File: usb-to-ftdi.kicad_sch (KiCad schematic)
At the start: 9 parts, among them J1 USB_OTG, J2 Conn_01x06, U1 AMS1117-3.3, U2 CH340C

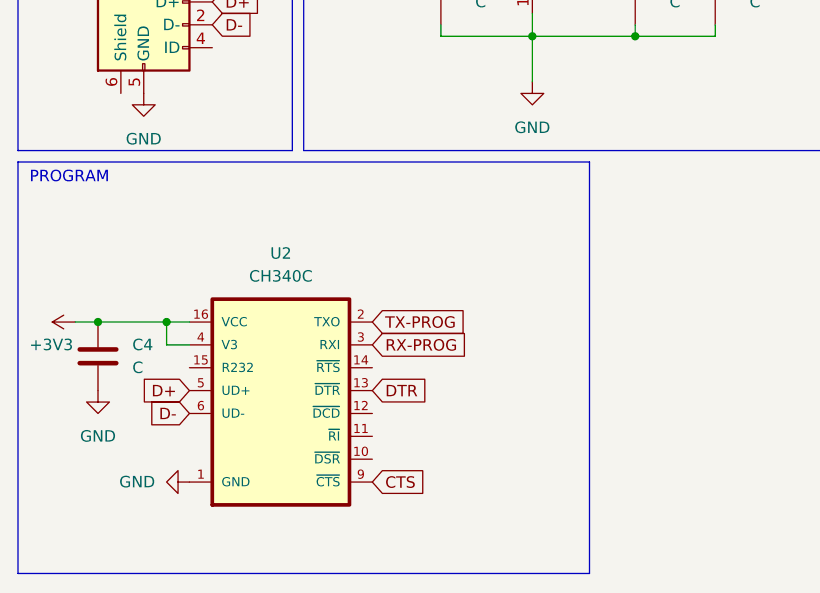
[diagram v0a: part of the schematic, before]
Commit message: add pcb + wiring
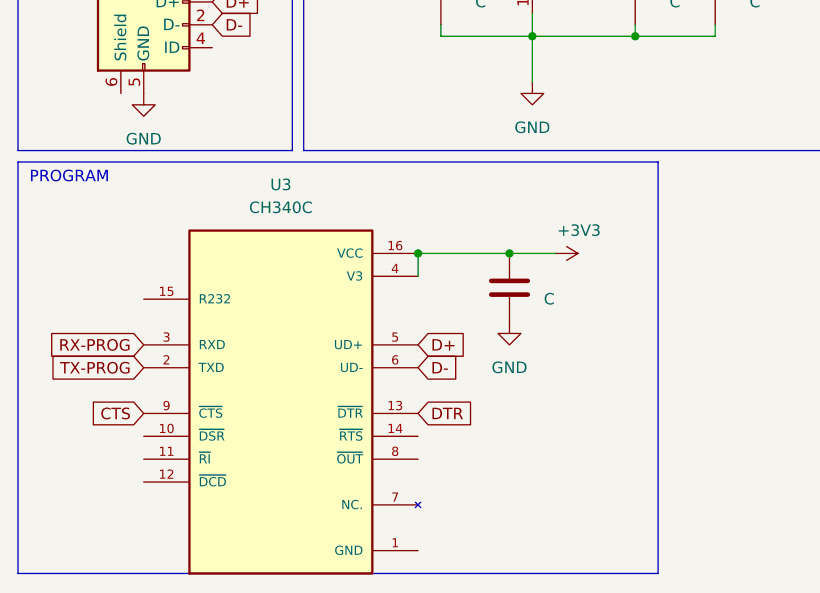
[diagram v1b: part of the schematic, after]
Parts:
- removed U2: CH340C, CH340C:SO016, symbol CH340C:CH340C
- added U3: CH340C, CH340C:SOIC127P600X180-16N, symbol CH340:CH340C
- J2: footprint (none) -> Connector_PinHeader_2.54mm:PinHeader_1x06_P2.54mm_Vertical
- JP1: footprint (none) -> Jumper:SolderJumper-3_P1.3mm_Bridged12_Pad1.0x1.5mm
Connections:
- net +3V3: now also U3.16 (VCC), U3.4 (V3)
- net CTS: now also U3.9 (~{CTS})
- net D+: now also U3.5 (UD+)
- net D-: now also U3.6 (UD-)
- net DTR: now also U3.13 (~{DTR})
- net RX-PROG: now also U3.3 (RXD)
- net TX-PROG: now also U3.2 (TXD)
